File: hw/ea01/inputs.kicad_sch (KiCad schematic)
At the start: 1 part, among them U9 74HC14

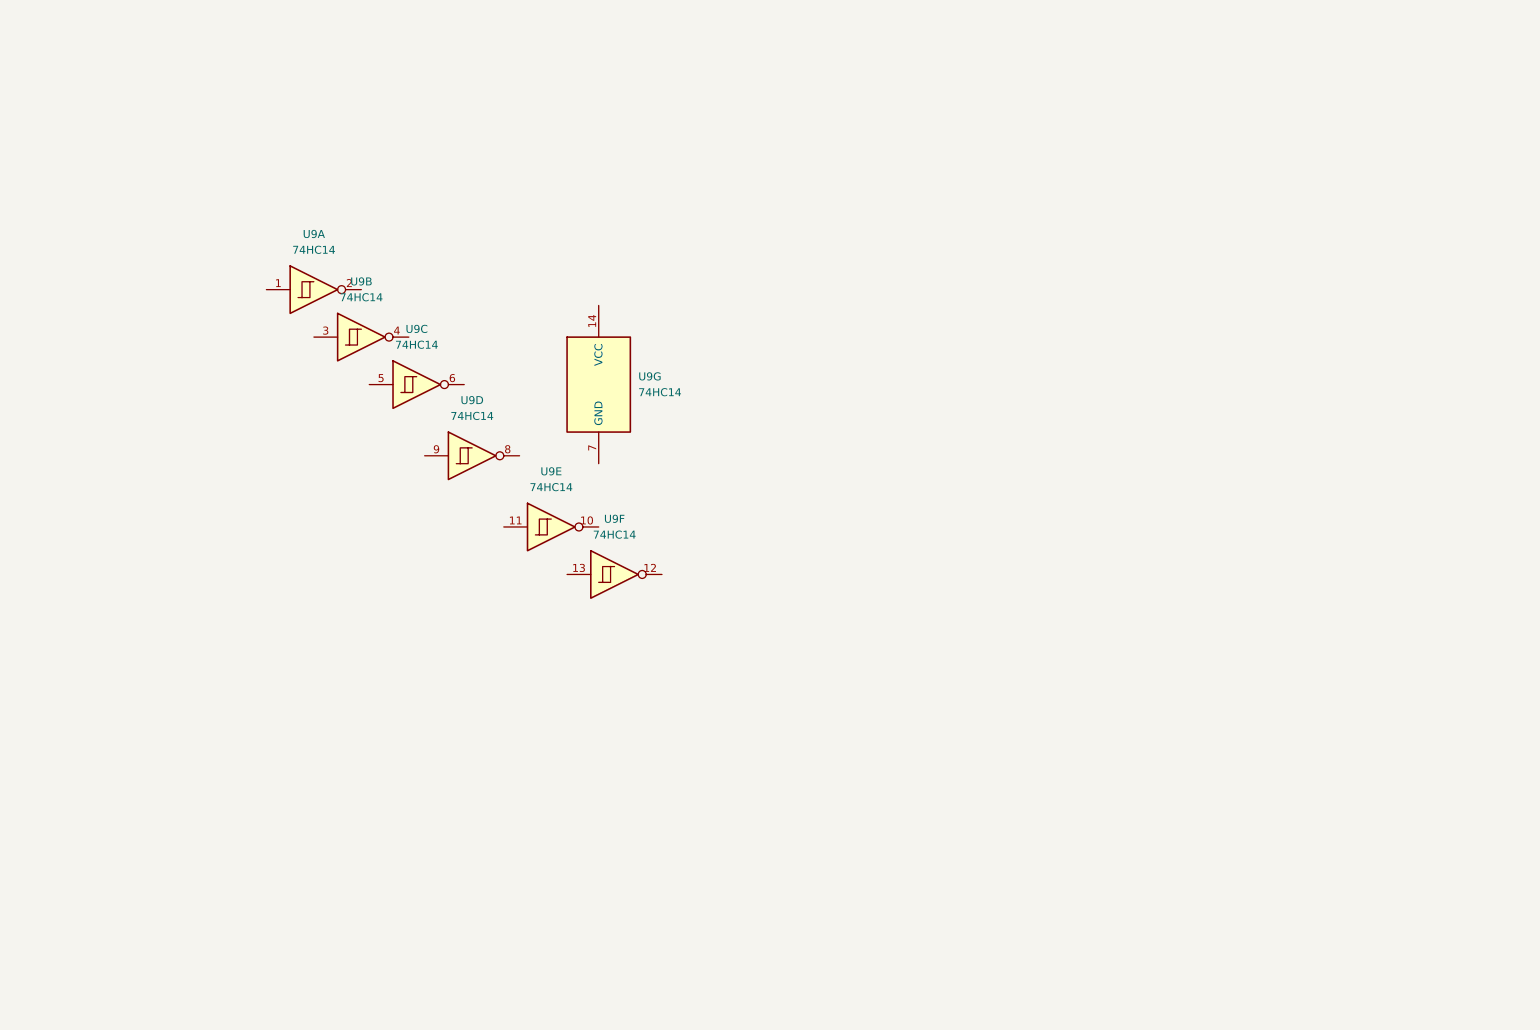
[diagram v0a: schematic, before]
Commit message: schmatic drawing continue...
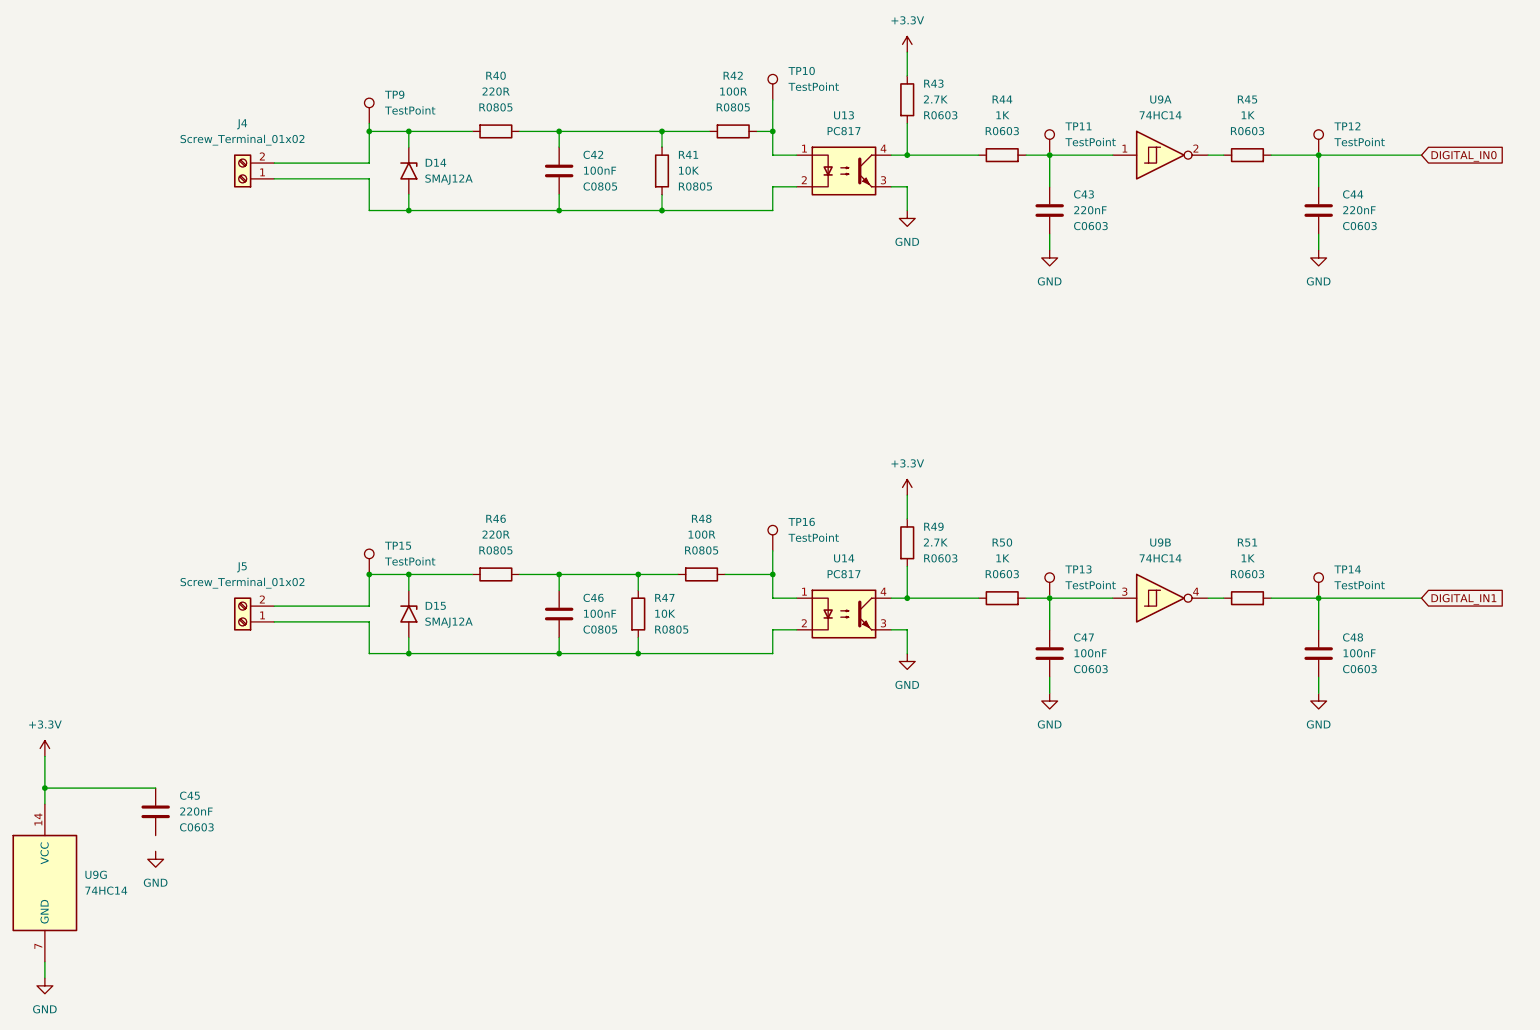
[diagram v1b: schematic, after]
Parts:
- removed unit 6 of U9
- removed unit 4 of U9
- removed unit 5 of U9
- removed unit 3 of U9
- added C42, C46: 100nF, Capacitor_SMD:C_0805_2012Metric, symbol Device:C
- added C43, C44, C45: 220nF, Capacitor_SMD:C_0603_1608Metric, symbol Device:C
- added C47, C48: 100nF, Capacitor_SMD:C_0603_1608Metric, symbol Device:C
- added D14, D15: SMAJ12A, Diode_SMD:D_SMA, symbol Diode:SMAJ24A
- added J4, J5: Screw_Terminal_01x02, TerminalBlock_RND:TerminalBlock_RND_205-00232_1x02_P5.08mm_Horizontal, symbol Connector:Screw_Terminal_01x02
- added R40, R46: 220R, Resistor_SMD:R_0805_2012Metric, symbol Device:R
- added R41, R47: 10K, Resistor_SMD:R_0805_2012Metric, symbol Device:R
- added R42, R48: 100R, Resistor_SMD:R_0805_2012Metric, symbol Device:R
- added R43, R49: 2.7K, Resistor_SMD:R_0603_1608Metric, symbol Device:R
- added R44, R45, R50, R51: 1K, Resistor_SMD:R_0603_1608Metric, symbol Device:R
- added TP10, TP11, TP12, TP13, TP14, TP15, TP16, TP9: TestPoint, TestPoint:TestPoint_Pad_D1.5mm, symbol Connector:TestPoint
- added U13, U14: PC817, Package_DIP:DIP-4_W7.62mm, symbol Isolator:PC817
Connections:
- net at U9.1: now also C43.1, R44.2, TP11.1
- net at U9.2: now also R45.1
- net at U9.3: now also C47.1, R50.2, TP13.1
- net at U9.4: now also R51.1
- net +3.3V: now reaches U9.14 (VCC)
- net +3.3V: now also C45.1, R43.1, R49.1
- net GND: now reaches U9.7 (GND)
- net GND: now also C43.2, C44.2, C47.2, C48.2, U13.3, U14.3
- new net: R48.1, TP16.1, U14.1
- new net: C46.2, D15.2 (A2), J5.1 (Pin_1), R47.2, U14.2
- new net: R49.2, R50.1, U14.4
- new net: C46.1, R46.1, R47.1, R48.2
- new net: D14.1 (A1), J4.2 (Pin_2), R40.2, TP9.1
- new net: C42.2, D14.2 (A2), J4.1 (Pin_1), R41.2, U13.2
- new net: D15.1 (A1), J5.2 (Pin_2), R46.2, TP15.1
- new net: R42.1, TP10.1, U13.1
- new net: C42.1, R40.1, R41.1, R42.2
- new net: R43.2, R44.1, U13.4
- new net DIGITAL_IN0: C44.1, R45.2, TP12.1
- new net DIGITAL_IN1: C48.1, R51.2, TP14.1
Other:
- moved on the sheet: U9A, U9B, U9G

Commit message: errors fix for comp fp
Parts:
- J4, J5: footprint TerminalBlock_RND:TerminalBlock_RND_205-00232_1x02_P5.08mm_Horizontal -> TerminalBlock:TerminalBlock_bornier-2_P5.08mm
- U9: footprint (none) -> Package_SO:SOIC-14_3.9x8.7mm_P1.27mm
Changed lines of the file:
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@@
 			)
 		)
-		(property "Footprint" ""
+		(property "Footprint" "Package_SO:SOIC-14_3.9x8.7mm_P1.27mm"
 			(at 207.01 50.8 0)
 			(effects
@@
 			)
 		)
-		(property "Footprint" "TerminalBlock_RND:TerminalBlock_RND_205-00232_1x02_P5.08mm_Horizontal"
+		(property "Footprint" "TerminalBlock:TerminalBlock_bornier-2_P5.08mm"
 			(at 59.69 125.73 0)
 			(effects
@@
 			)
 		)
-		(property "Footprint" "TerminalBlock_RND:TerminalBlock_RND_205-00232_1x02_P5.08mm_Horizontal"
+		(property "Footprint" "TerminalBlock:TerminalBlock_bornier-2_P5.08mm"
 			(at 59.69 54.61 0)
 			(effects
@@
 			)
 		)
-		(property "Footprint" ""
+		(property "Footprint" "Package_SO:SOIC-14_3.9x8.7mm_P1.27mm"
 			(at 207.01 121.92 0)
 			(effects
@@
 			)
 		)
-		(property "Footprint" ""
+		(property "Footprint" "Package_SO:SOIC-14_3.9x8.7mm_P1.27mm"
 			(at 27.94 167.64 0)
 			(effects
